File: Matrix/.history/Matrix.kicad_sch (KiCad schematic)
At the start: 146 parts, among them J1 Conn_01x08, Q1 2N2219, Q10 2N2219, Q11 2N2219, Q12 2N2219, Q13 2N2219, Q14 2N2219, Q15 2N2219, Q16 2N2219, Q2 2N2219, Q3 2N2219, Q4 2N2219, Q5 2N2219, Q6 2N2219, Q7 2N2219, Q8 2N2219, Q9 2N2219, U1 74HC138, U10 ESP32-S3, U2 74HC574N, U3 74HC574N, U4 74HC574N, U5 74HC574N, U6 74HC574N, U7 74HC574N, U8 74HC574N, U9 74HC574N

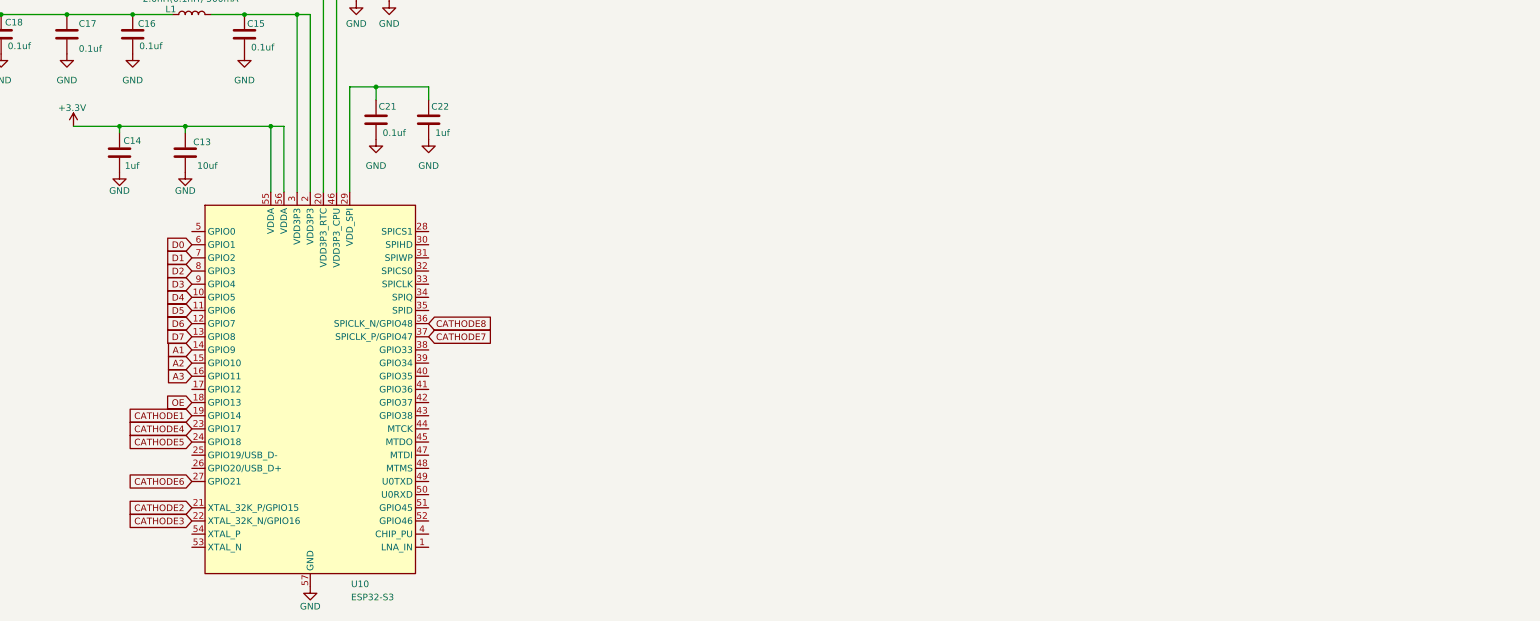
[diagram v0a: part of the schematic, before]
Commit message: Update Matrix.kicad_sch
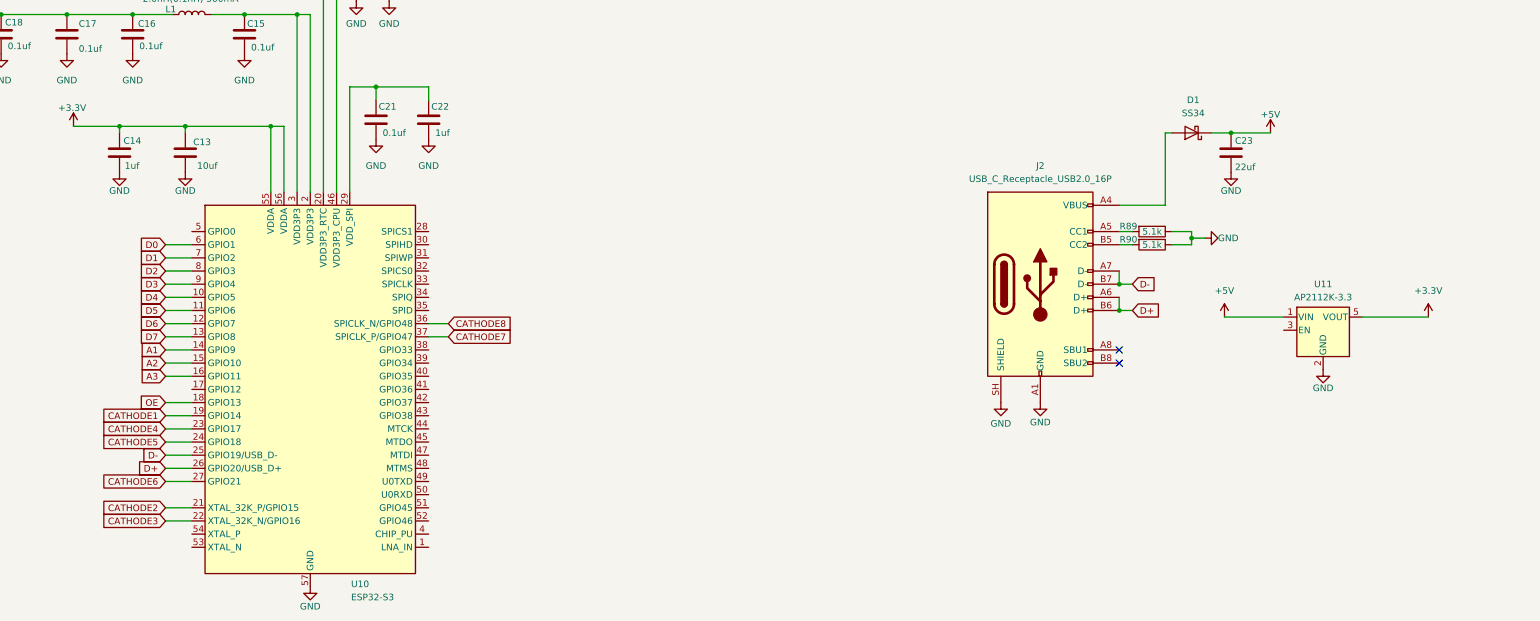
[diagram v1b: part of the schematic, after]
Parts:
- added C23: 22uf, symbol Device:C
- added D1: SS34, Diode_SMD:D_SMA, symbol Diode:SS34
- added J2: USB_C_Receptacle_USB2.0_16P, symbol Connector:USB_C_Receptacle_USB2.0_16P
- added R89, R90: 5.1k, symbol Device:R
- added U11: AP2112K-3.3, Package_TO_SOT_SMD:SOT-23-5, symbol Regulator_Linear:AP2112K-3.3
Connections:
- net +3.3V: now also U11.5 (VOUT)
- net +5V: now also C23.1, D1.1 (K), U11.1 (VIN)
- net GND: now also C23.2, J2.A1 (GND), J2.A12 (GND), J2.B1 (GND), J2.B12 (GND), J2.SH (SHIELD), R89.1, R90.1, U11.2 (GND)
- net D-: now reaches U10.25 (GPIO19/USB_D-)
- net D-: now also J2.A7 (D-), J2.B7 (D-)
- net D+: now reaches U10.26 (GPIO20/USB_D+)
- net D+: now also J2.A6 (D+), J2.B6 (D+)
- new net: J2.B5 (CC2), R90.2
- new net: J2.A5 (CC1), R89.2
- new net: D1.2 (A), J2.A4 (VBUS), J2.A9 (VBUS), J2.B4 (VBUS), J2.B9 (VBUS)
- no-connect marks 0 -> 2
